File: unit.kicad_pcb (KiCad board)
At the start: 4 copper layers, 45 x 30 mm, 81 parts, among them J3 Micro_SD_Card_Det1, J4 Conn_01x03_Socket, J5 SWD, Q1 AO3400A, U1 RT9013, U2 W25Q128JVS, U3 TPS61040DBV, U5 MPU-6050, U6 STM32F407VETx, Y1 8MHz

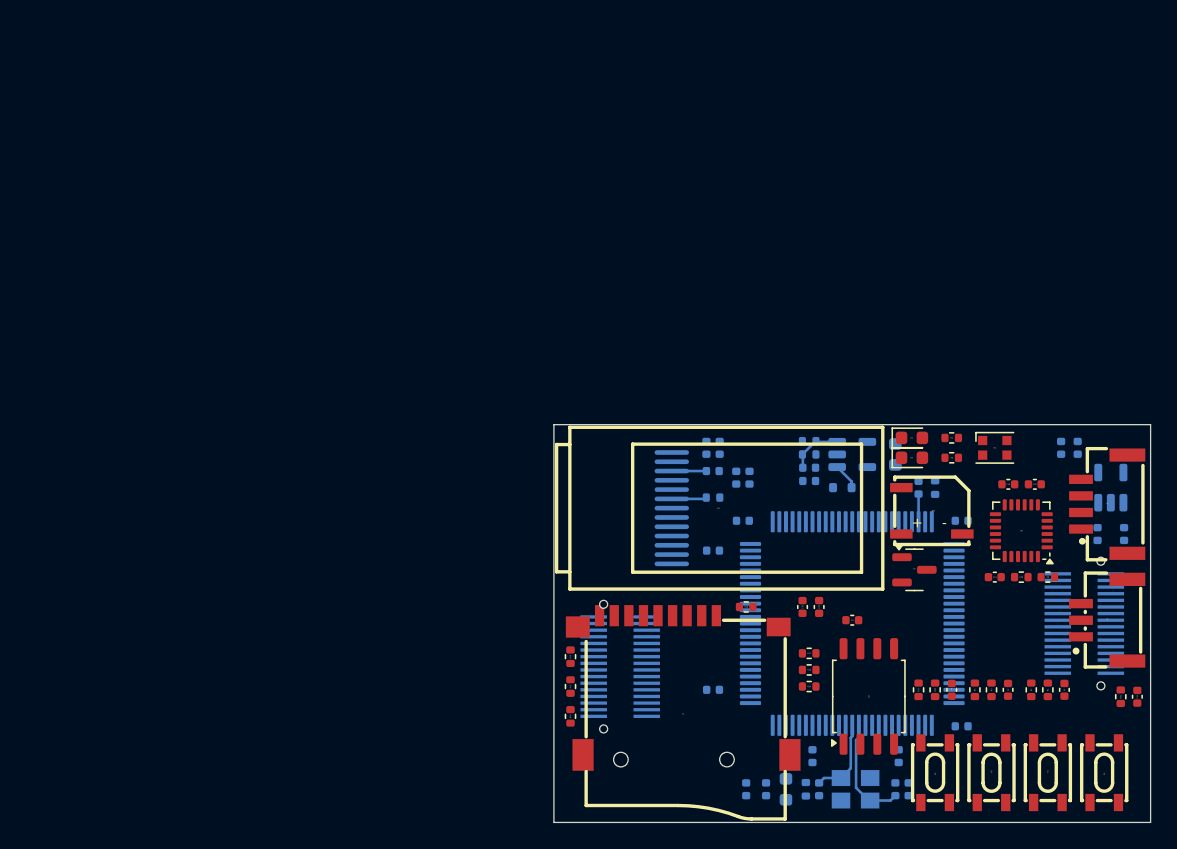
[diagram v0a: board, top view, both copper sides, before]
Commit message: update v1.0
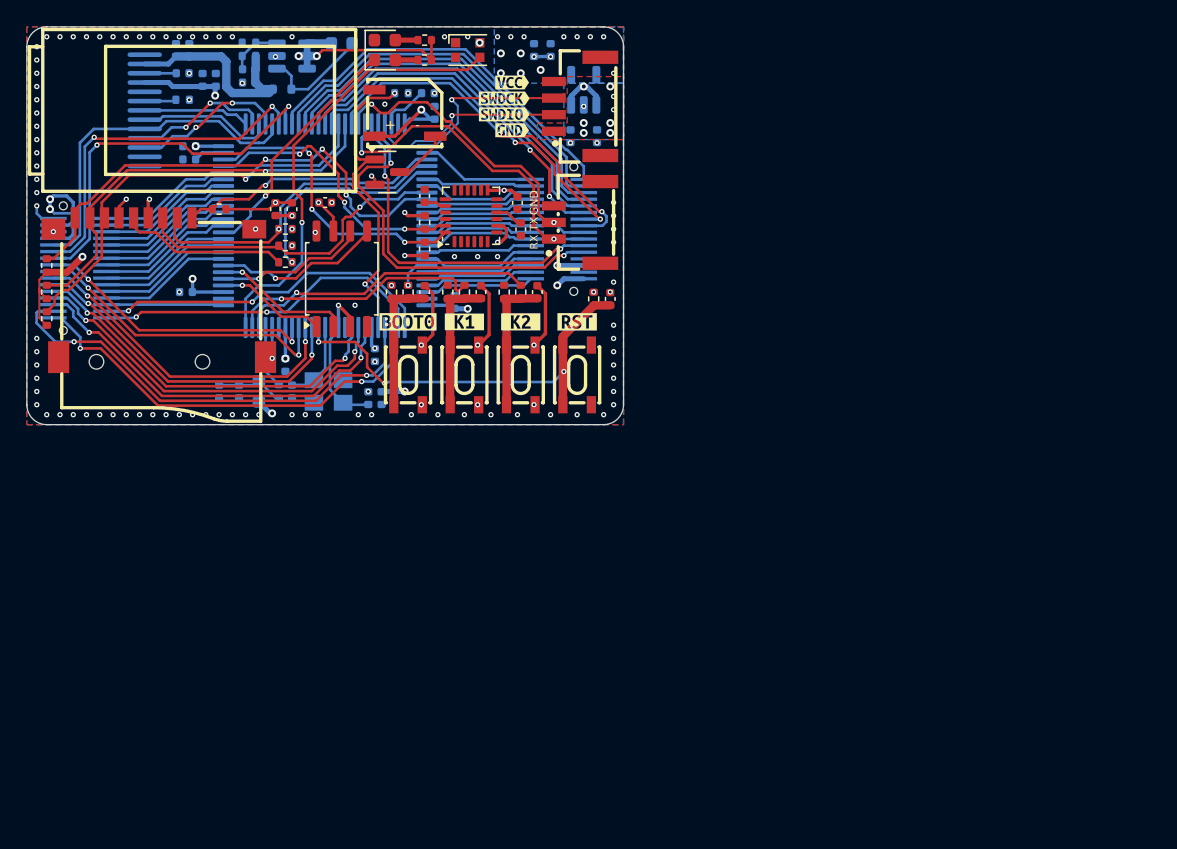
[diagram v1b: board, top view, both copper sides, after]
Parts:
- added kibuzzard-66CADDA5: G***, kibuzzard-66CADDA5, F.Cu at (125.8, 76.4)
- added kibuzzard-66CADDDA: G***, kibuzzard-66CADDDA, F.Cu at (117.3, 76.4)
- added kibuzzard-66CADE49: G***, kibuzzard-66CADE49, F.Cu at (121.6, 76.4)
- added kibuzzard-66CADE69: G***, kibuzzard-66CADE69, F.Cu at (113.1, 76.4)
- added kibuzzard-66CADF13: G***, kibuzzard-66CADF13, F.Cu at (120.3, 60.7)
- added kibuzzard-66CADF25: G***, kibuzzard-66CADF25, F.Cu at (120.3, 59.5)
- added kibuzzard-66CADF6D: G***, kibuzzard-66CADF6D, F.Cu at (121.0, 58.3)
- added kibuzzard-66CADF7A: G***, kibuzzard-66CADF7A, F.Cu at (121.0, 61.9)
- moved R9 53.1 mm to (114.3, 70.9), turned to 90 degrees
- moved R10 52.4 mm to (114.3, 68.9), turned to -90 degrees
- moved L1 52.0 mm to (108.1, 55.4), turned to 0 degrees
- moved C8 51.8 mm to (101.1, 57.3)
- moved C9 51.8 mm to (101.1, 58.3)
- moved D4 51.8 mm to (103.6, 58.8)
- moved R7 51.8 mm to (101.1, 56.3)
- moved R8 51.8 mm to (101.1, 55.3)
- moved U3 51.8 mm to (104.3, 56.3)
- moved C24 51.7 mm to (114.3, 66.9), turned to -90 degrees
- moved R14 50.8 mm to (85.8, 74.1)
- moved R16 50.8 mm to (103.8, 70.6), turned to 180 degrees
- moved R17 50.8 mm to (103.8, 69.4), turned to 180 degrees
- moved R20 50.8 mm to (103.8, 71.9)
- moved C3 50.7 mm to (106.8, 67.4)
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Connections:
- J1 pad 1: /PA3 -> /PE4
- J1 pad 10: /PE11 -> /PD10
- J1 pad 11: /PE12 -> /PD9
- J1 pad 12: /PE13 -> /OLED_DC
- J1 pad 13: /PE14 -> VCC
- J1 pad 14: /PE15 -> GND
- J1 pad 17: VCC -> /PE15
- J1 pad 18: GND -> /PE14
- J1 pad 19: /OLED_DC -> /PE13
- J1 pad 2: /PC4 -> /PE5
- J1 pad 20: /PD9 -> /PE12
- J1 pad 21: /PD10 -> /PE11
- J1 pad 22: /PD11 -> /PE10
- J1 pad 23: /PD12 -> /PE9
- J1 pad 24: /PD13 -> /PE8
- J1 pad 25: /PD14 -> /PE7
- J1 pad 26: /PD15 -> /PB1
- J1 pad 27: /PC6 -> /PB0
- J1 pad 28: /PC7 -> /PC5
- J1 pad 29: /PA8 -> /PC4
- J1 pad 3: /PC5 -> /PC13
- J1 pad 30: /PA11 -> /PA3
- J1 pad 31: /PA12 -> /PE2
- J1 pad 32: /PA15 -> /PE3
- J1 pad 4: /PB0 -> /PC14
- J1 pad 5: /PB1 -> /PC15
- J1 pad 6: /PE7 -> /PC0
- J1 pad 7: /PE8 -> /PC1
- J1 pad 8: /PE9 -> /PC2
- J1 pad 9: /PE10 -> /PC3
- J2 pad 1: /PA9 -> /PD11
- J2 pad 10: /PB4 -> /PA10
- J2 pad 11: /PB5 -> /PA11
- J2 pad 12: /PB6 -> /PA12
- J2 pad 13: /PB7 -> GND
- J2 pad 14: /PB8 -> VCC
- J2 pad 15: /PB9 -> GND
- J2 pad 17: /PE0 -> /PE1
- J2 pad 18: /PE1 -> /PE0
- J2 pad 19: /PE2 -> /PB9
- J2 pad 2: /PA10 -> /PD12
- J2 pad 20: /PE3 -> /PB8
- J2 pad 21: /PE4 -> /PB7
- J2 pad 22: /PE5 -> /PB6
- J2 pad 23: /PC13 -> /PB5
- J2 pad 24: /PC14 -> /PB4
- J2 pad 25: /PC15 -> /PB3
- J2 pad 26: /PC0 -> /PD7
- J2 pad 27: /PC1 -> /PD6
- J2 pad 28: /PC2 -> /PD5
- J2 pad 29: /PC3 -> /PD4
- J2 pad 3: /PD0 -> /PD13
- J2 pad 30: GND -> /PD1
- J2 pad 31: VCC -> /PD0
- J2 pad 32: GND -> /PA15
- J2 pad 4: /PD1 -> /PD14
- J2 pad 5: /PD4 -> /PD15
- J2 pad 6: /PD5 -> /PC6
- J2 pad 7: /PD6 -> /PC7
- J2 pad 8: /PD7 -> /PA8
- J2 pad 9: /PB3 -> /PA9
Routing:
- net +3V3: track 0.00 -> 90.1 mm, vias 0 -> 35
- net /PD3: track 0.00 -> 36.9 mm, vias 0 -> 3
- net /PE5: track 0.00 -> 34.6 mm, vias 0 -> 2
- net /PA2: track 0.00 -> 33.4 mm, vias 0 -> 1
- net /PE4: track 0.00 -> 32.2 mm, vias 0 -> 2
- net /NRST: track 0.00 -> 31.5 mm, vias 0 -> 3
- net /PC8: track 0.00 -> 30.9 mm, vias 0 -> 1
- net /PC9: track 0.00 -> 30.5 mm, vias 0 -> 1
- net /PC13: track 0.00 -> 30.0 mm, vias 0 -> 2
- net /PD12: track 0.00 -> 29.5 mm
- net /PD11: track 0.00 -> 29.5 mm
- net /PC14: track 0.00 -> 29.3 mm, vias 0 -> 2
- net /PA12: track 0.00 -> 28.9 mm, vias 0 -> 2
- net /PD13: track 0.00 -> 28.9 mm
- net /PC15: track 0.00 -> 28.5 mm, vias 0 -> 2
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- added copper zone on B.Cu, net +3V3
- added copper zone on In1.Cu, net +3V3
- added copper zone on B.Cu, net GND
- added copper zone on F.Cu, net GND
- added copper zone on In2.Cu, net GND
- added copper zone on B.Cu, net VCC
- added copper zone on F.Cu, net VCC
- added copper zone on In1.Cu, net VCC
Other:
- outline, holes or cut-outs redrawn
- board text added: "GND"
- board text added: "RX"
- board text added: "TX"
